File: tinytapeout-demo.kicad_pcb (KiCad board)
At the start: 4 copper layers, 99.5 x 78 mm, 319 parts, among them J1 Conn_01x06, J10 Conn_01x02, J11 Conn_01x06, J12 613012243121, J13 613012243121, J14 613012243121, J16 2x20_P2.54mm_Pinheader, J17 Conn_01x03, J18 2x20_P2.54mm_Pinheader, J19 Conn_01x02, J2 Conn_01x04, J20 USB_C, J3 613012243121, J4 TT06_BREAKOUT_REVA, J5 613012243121, J6 613012243121, J7 Conn_01x02, J8 Conn_01x03, J9 Conn_01x16, Q1 DMN2005K, SW1 434121025816, SW2 434121025816, SW3 434121025816, SW4 193-8MSR, U1 157112V12700, U2 TLV1117LV33, U3 AP2112K-1.8, U5 W25Q32JVSS, U6 RP2040, Y1 12.0MHz

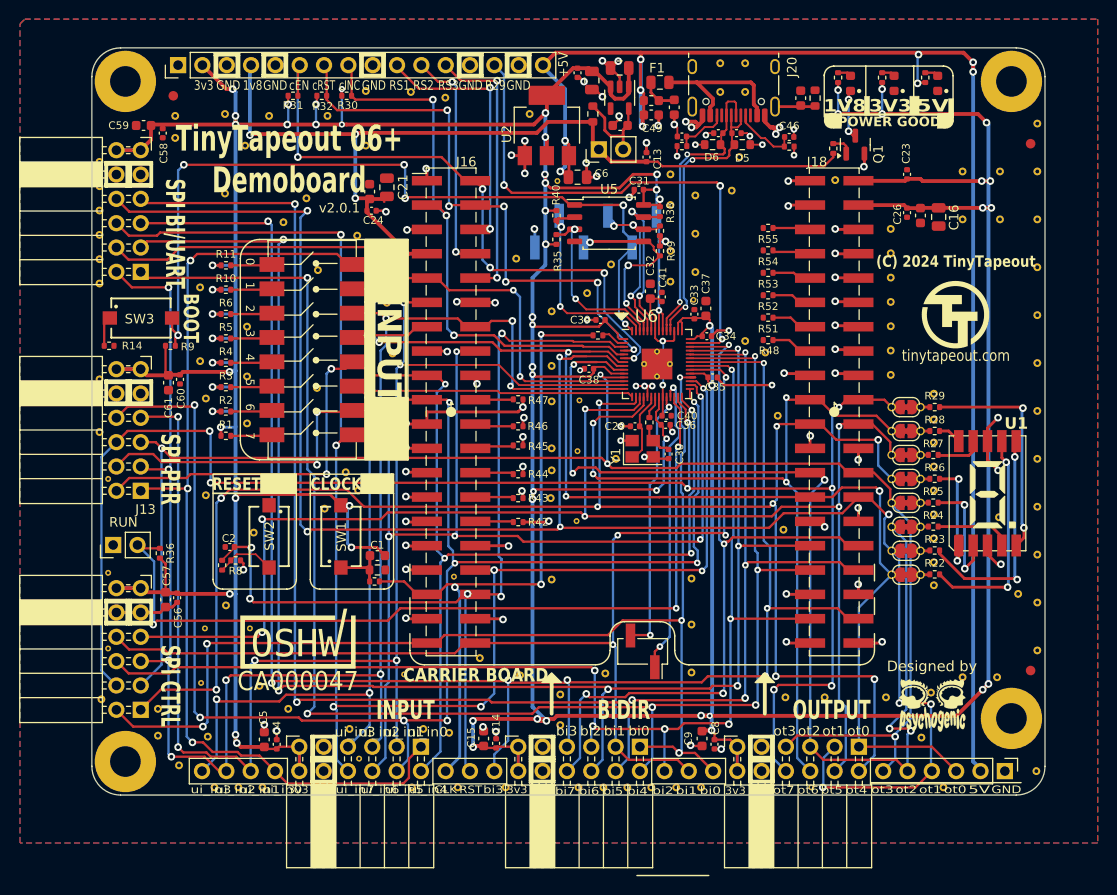
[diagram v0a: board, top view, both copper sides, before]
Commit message: the great relabelling
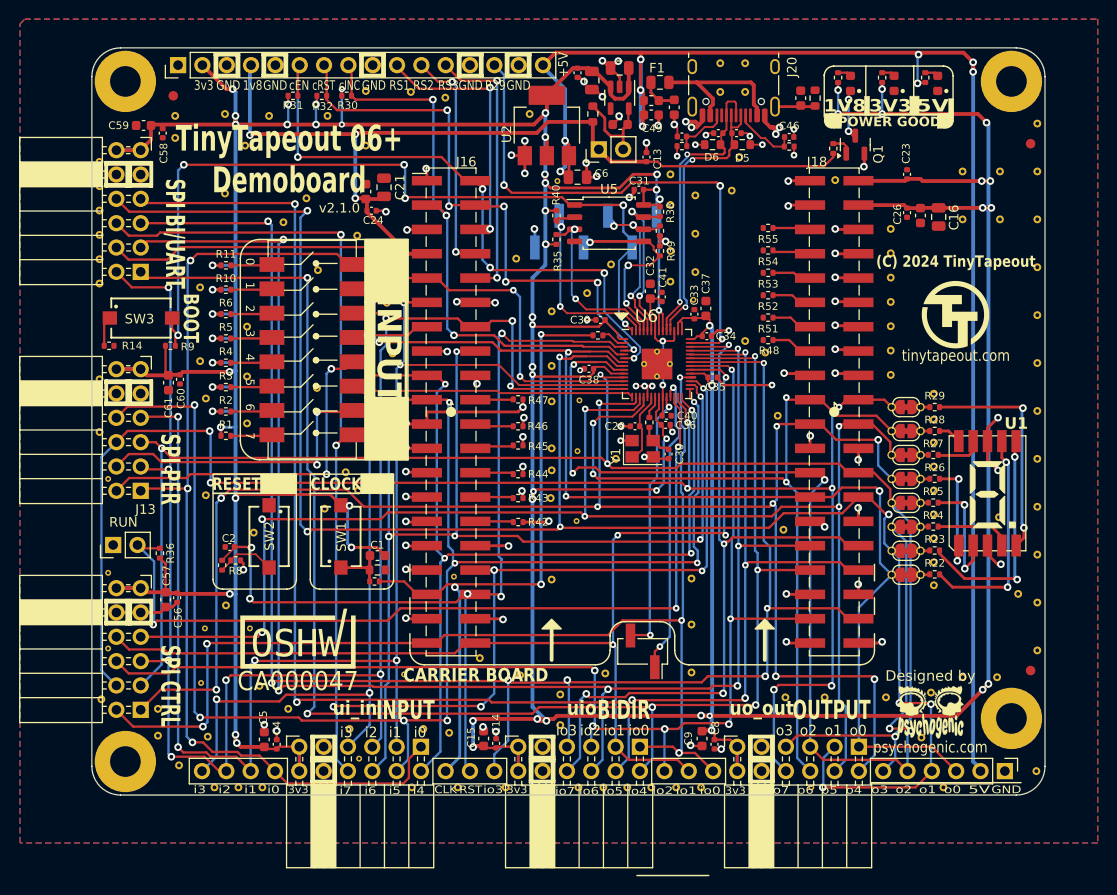
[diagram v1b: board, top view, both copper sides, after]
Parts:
- R42, R43, R44, R45, R46, R47, R48, R51, R52, R53, R54, R55: value 10k -> 1M
- moved TTLOGO2 1.79 mm to (147.6, 76.0)
- moved Z2ALOGO2 1.79 mm to (127.5, 75.9)
- moved OSHWLOGO2 1.00 mm to (87.5, 67.5)
- moved PSYLOGO1 1.00 mm to (87.8, 77.0)
- moved PSYLOGO2 0.73 mm to (147.0, 122.8)
- moved C25 0.40 mm to (88.1, 68.5)
- moved C21 0.30 mm to (90.0, 68.0)
- moved C11 0.10 mm to (114.7, 61.5)
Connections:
- J16 pad 1: unconnected-(J16-Pad1) -> GND
- J18 pad 1: unconnected-(J18-Pad1) -> uo_out6
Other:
- board text added: "RP2040 upgrades: * Hold BOOT button * Connect to USB * Release BOOT Should see an RPI-RP2 drive. Copy UF2 file over, that's it."
- board text added: "i0"
- board text added: "i1"
- board text added: "i2"
- board text added: "i3"
- board text added: "i4"
- board text added: "i5"
- board text added: "i6"
- board text added: "i7"
- board text added: "io0"
- board text added: "io1"
- board text added: "io2"
- board text added: "io3"
- board text added: "io4"
- board text added: "io5"
- board text added: "io6"
- board text added: "io7"
- board text added: "o0"
- board text added: "o1"
- board text added: "o2"
- board text added: "o3"
- board text added: "o4"
- board text added: "o5"
- board text added: "o6"
- board text added: "o7"
- board text added: "ui_in"
- board text added: "uio"
- board text added: "uo_out"
- board text added: "v2.1.0"
- board text removed: "RP2040 upgrades: * Hold BOOT button * Connect to USB * Release BOOT Should see an RPI-RP2 drive. Copy UF2 file over, done."
- board text removed: "bi0"
- board text removed: "bi1"
- board text removed: "bi2"
- board text removed: "bi3"
- board text removed: "bi4"
- board text removed: "bi5"
- board text removed: "bi6"
- board text removed: "bi7"
- board text removed: "ot0"
- board text removed: "ot1"
- board text removed: "ot2"
- board text removed: "ot3"
- board text removed: "ot4"
- board text removed: "ot5"
- board text removed: "ot6"
- board text removed: "ot7"
- board text removed: "ui_in0"
- board text removed: "ui_in1"
- board text removed: "ui_in2"
- board text removed: "ui_in3"
- board text removed: "ui_in4"
- board text removed: "ui_in5"
- board text removed: "ui_in6"
- board text removed: "ui_in7"
- board text removed: "v2.0.1"
